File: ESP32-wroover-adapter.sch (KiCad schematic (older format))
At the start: 20 parts, among them J1 USB_OTG, J2 Screw_Terminal_01x03, J3 Screw_Terminal_01x03, J4 Screw_Terminal_01x03, J5 Screw_Terminal_01x03, J6 Conn_01x20, J7 Conn_01x07, J8 Screw_Terminal_01x02, Q1 Q_NPN_BCE, Q2 Q_NPN_BCE, Q3 Q_PMOS_DGS, SW1 SW_Push, U1 ESP32-WROVER, U2 ap2112, U3 BME280, U4 CP2104

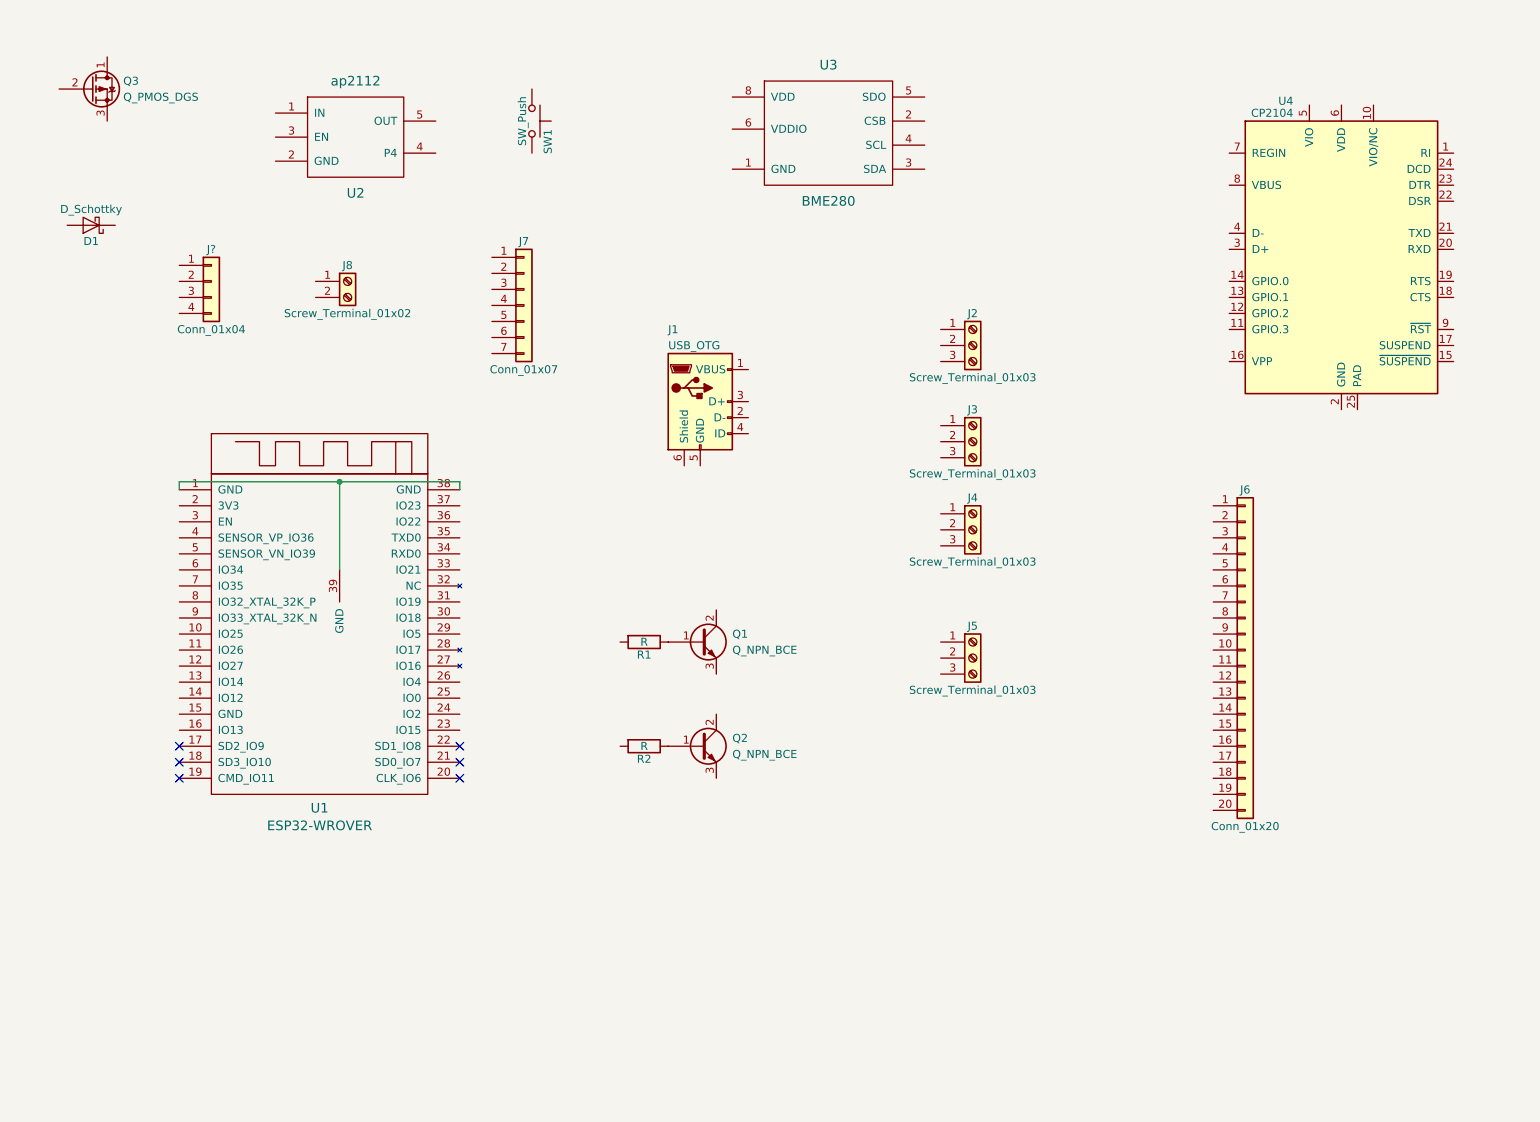
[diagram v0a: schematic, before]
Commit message: update
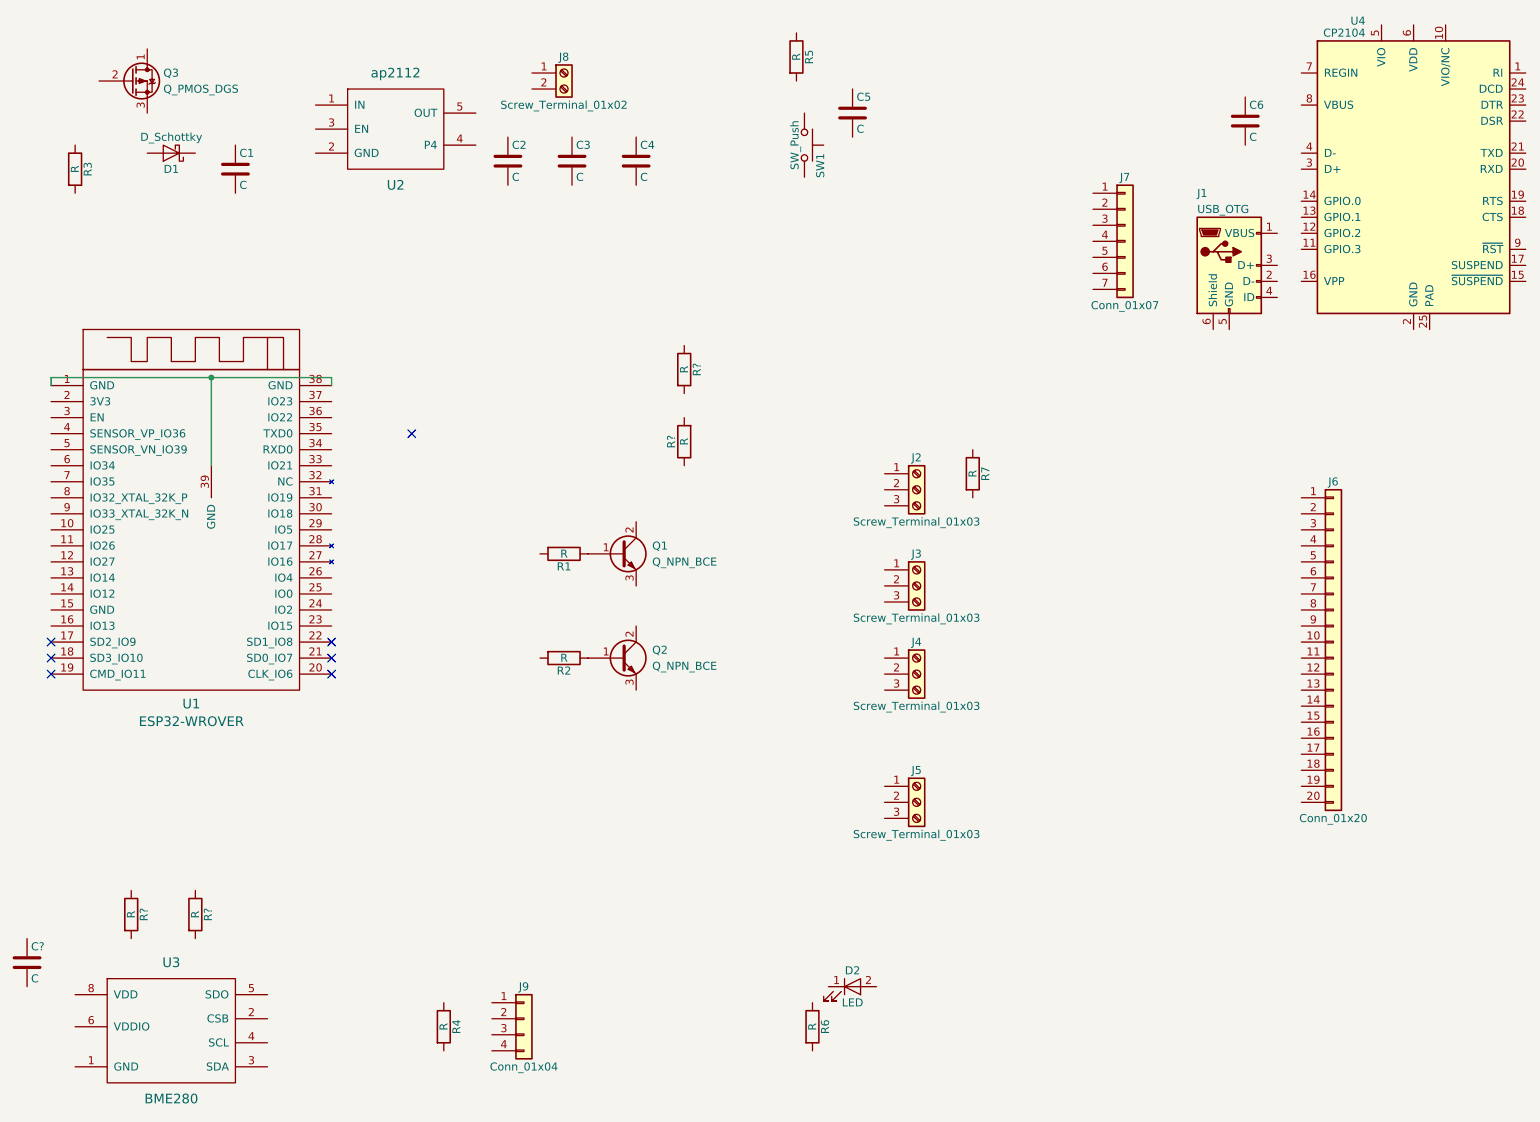
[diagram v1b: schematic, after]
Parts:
- added C1, C2, C3, C4, C5, C6: C, Capacitors_SMD:C_0603, symbol C
- added C?: C, symbol C
- added D2: LED, LEDs:LED_0603, symbol LED
- added R3, R4, R5, R6, R7: R, Resistors_SMD:R_0603, symbol R
- added R? (x4): R, symbol R
- J9: renamed from J?; footprint (none) -> Pin_Headers:Pin_Header_Straight_1x04_Pitch2.54mm
- R1, R2: footprint Resistors_SMD:R_0805 -> Resistors_SMD:R_0603
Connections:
- no-connect marks 6 -> 7
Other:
- moved on the sheet: D1, J1, J2, J3, J4, J5, J6, J7, J8, J9, Q1, Q2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
